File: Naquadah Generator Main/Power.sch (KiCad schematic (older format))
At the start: 12 parts, among them J10 Power Board Conn, J9 Power_Conn, Q1 30V 5A

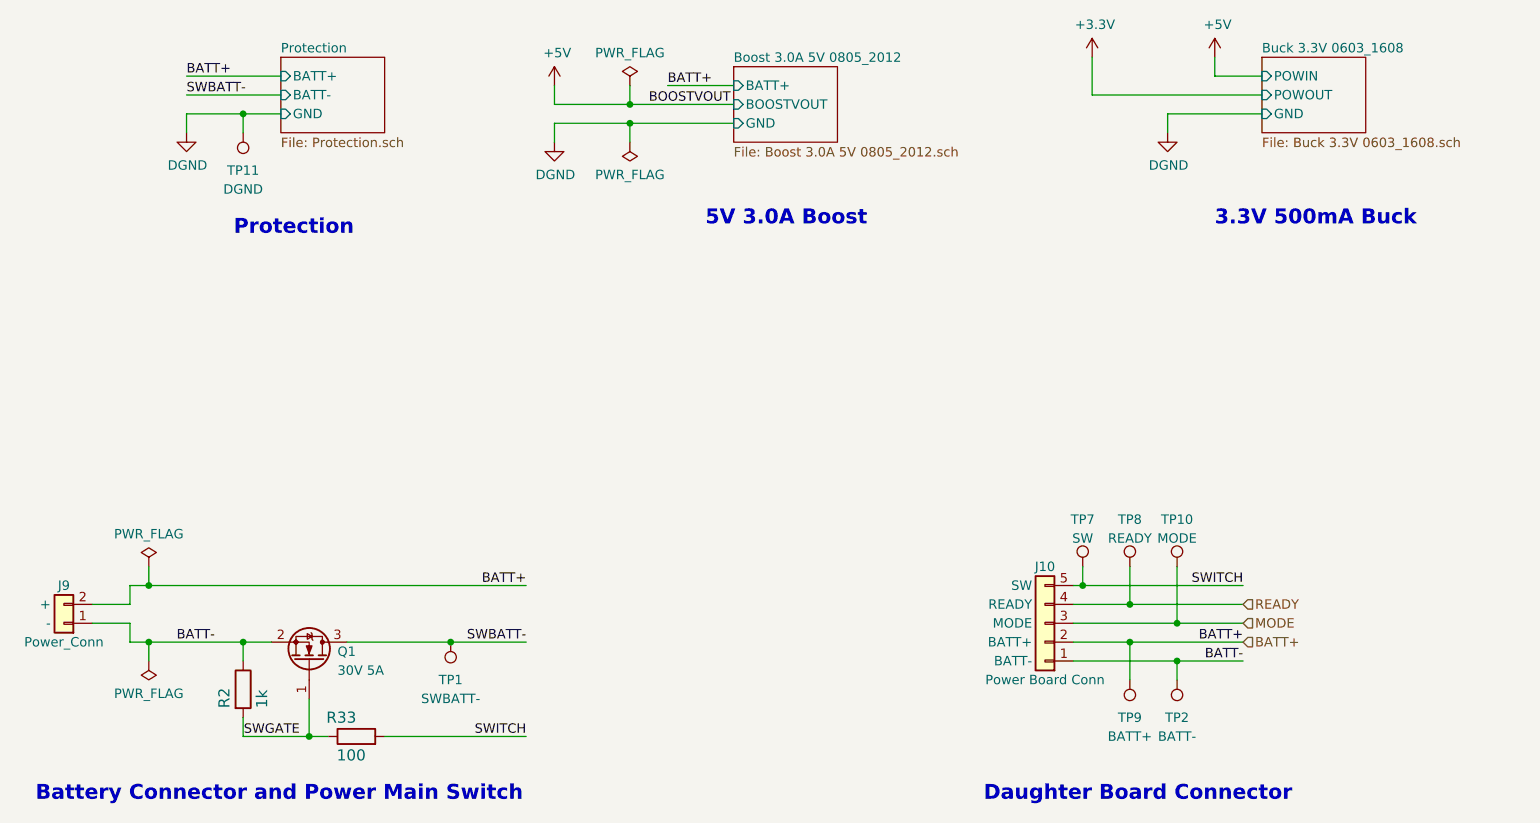
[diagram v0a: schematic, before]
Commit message: Added level shifter, moved user interface connector location
Added level shifter, moved user interface connector location
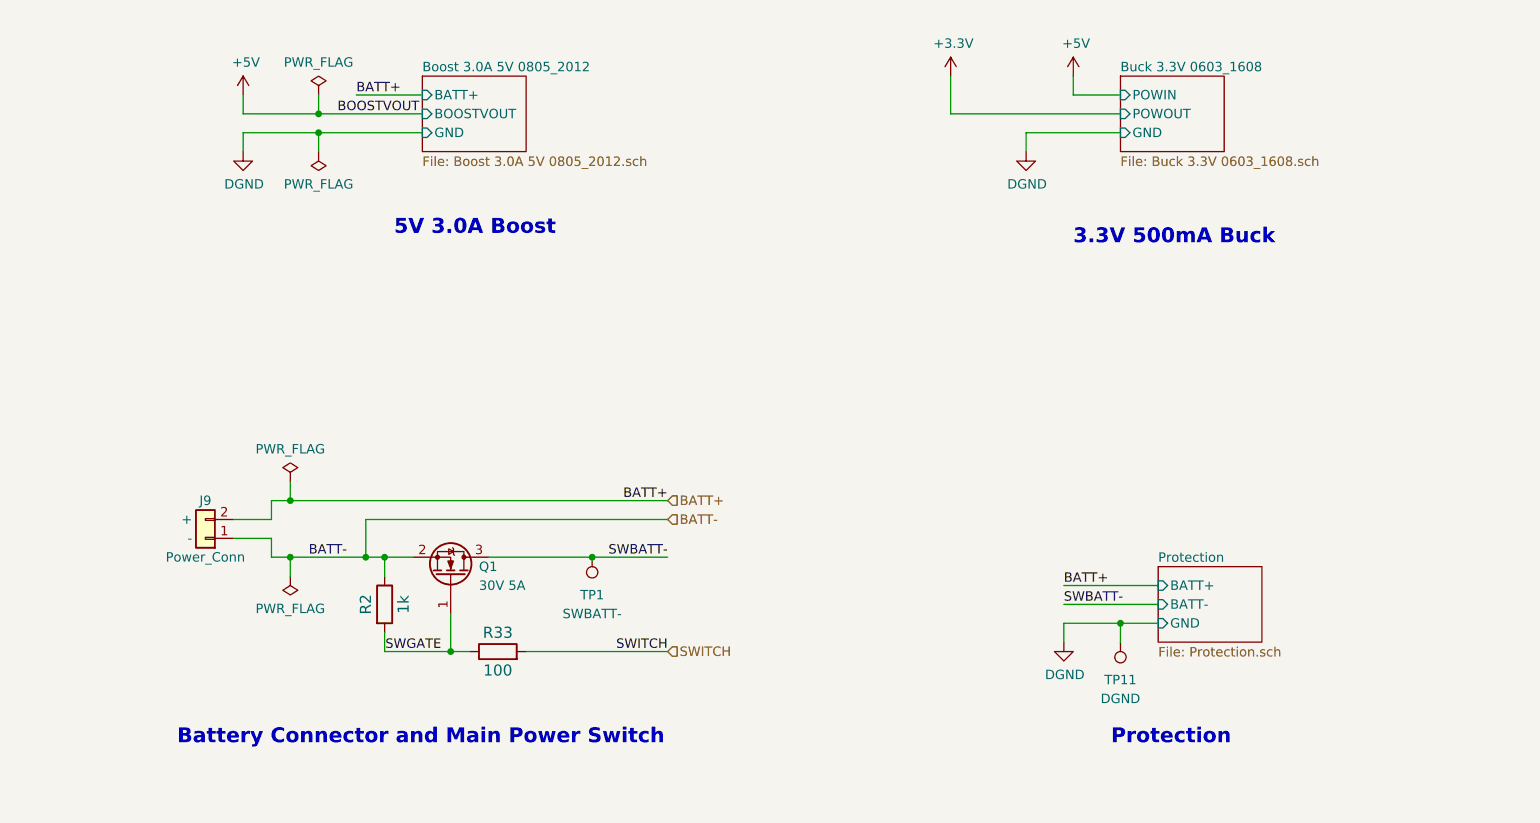
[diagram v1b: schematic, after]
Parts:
- removed J10: Power Board Conn, Naquadah_Generator:Daughter_Board_Vert_5_Pin_JST_Conn, symbol Naquadah_Generator:Power_Daughter_5_Pin_Conn
- removed TP10, TP2, TP7, TP8, TP9: TestPoint, Frequently_Used_LE:Pad_2.5-2.5, symbol Frequently_Used_LE:TestPoint_1
- R2: footprint Frequently_Used_LE:0805_2012Metric_HandSolder -> Frequently_Used_LE:0805_2012Metric
- R33: footprint Frequently_Used_LE:0805_2012Metric_HandSolder -> Frequently_Used_LE:0805_2012Metric; Description 1 kOhms ±1% 0.25W, 1/4W Chip Resistor 1206 (3216 Metric) -> 100 Ohms ±1% 0.25W, 1/4W Chip Resistor 0805 (2012 Metric) A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; Manufacturer Part No. RK73H2ATTD1001F -> RK73H2ATTD1000F; Source Part No. 2019-RK73H2ATTD1001FCT-ND -> 2019-RK73H2ATTD1000FCT-ND
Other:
- note added: "Battery Connector and Main Power Switch"
- note removed: "Battery Connector and Power Main Switch"
- note removed: "Daughter Board Connector"
- moved on the sheet: J9, Q1, R2, R33, TP1, TP11

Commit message: Switched to 0603_1608M size for passives
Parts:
- J9: symbol Connectors_LE:Power_Conn -> Connector_LE:Power_Conn; Description (none) -> Battery Holder (Open) 18650 1 Cell SMD (SMT) Tab; Manufacturer Name (none) -> Keystone Electronics; Manufacturer Part No. (none) -> 1042; Source (none) -> Digikey; Source Part No. (none) -> 36-1042-ND
- R2: footprint Frequently_Used_LE:0805_2012Metric -> Frequently_Used_LE:0603_1608Metric; Description 1 kOhms ±1% 0.25W, 1/4W Chip Resistor 1206 (3216 Metric) -> 1 kOhms ±1% 0.25W, 1/4W Chip Resistor 0603 (1608 Metric) Au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; Manufacturer Name KOA Speer Electronics, Inc. -> Rohm Semiconductor; Manufacturer Part No. RK73H2ATTD1001F -> ESR03EZPF1001; Source Part No. 2019-RK73H2ATTD1001FCT-ND -> RHM1.00KADCT-ND
- R33: footprint Frequently_Used_LE:0805_2012Metric -> Frequently_Used_LE:0603_1608Metric; Description 100 Ohms ±1% 0.25W, 1/4W Chip Resistor 0805 (2012 Metric) A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 -> 100 Ohms ±1% 0.25W, 1/4W Chip Resistor 0603 (1608 Metric) A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; Manufacturer Name KOA Speer Electronics, Inc. -> Panasonic Electronic Components; Manufacturer Part No. RK73H2ATTD1000F -> ERJ-PA3F1000V; Source Part No. 2019-RK73H2ATTD1000FCT-ND -> P100BYCT-ND
- TP1, TP11: Description None -> Test point
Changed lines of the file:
@@
 $Descr A 11000 8500
 encoding utf-8
-Sheet 10 17
+Sheet 10 18
 Title "Li-ion 3A Boost 1A Charge Protect"
 Date ""
@@
 F 0 "R33" V 4000 5250 59  0000 C CNN
 F 1 "100" V 3800 5250 59  0000 C CNN
-F 2 "Frequently_Used_LE:0805_2012Metric" H 3900 5250 50  0001 C CNN
-F 3 "http://www.koaspeer.com/pdfs/RK73H.pdf" H 3900 5250 50  0001 C CNN
-F 4 "100 Ohms ±1% 0.25W, 1/4W Chip Resistor 0805 (2012 Metric) Automotive AEC-Q200, Moisture Resistant Thick Film" H 3900 5250 50  0001 C CNN "Description"
-F 5 "2019-RK73H2ATTD1000FCT-ND" H 3900 5250 50  0001 C CNN "Source Part No."
-F 6 "RK73H2ATTD1000F" H 3900 5250 50  0001 C CNN "Manufacturer Part No."
-F 7 "KOA Speer Electronics, Inc." H 3900 5250 50  0001 C CNN "Manufacturer Name"
+F 2 "Frequently_Used_LE:0603_1608Metric" H 3900 5250 50  0001 C CNN
+F 3 "https://industrial.panasonic.com/cdbs/www-data/pdf/RDO0000/AOA0000C331.pdf" H 3900 5250 50  0001 C CNN
+F 4 "100 Ohms ±1% 0.25W, 1/4W Chip Resistor 0603 (1608 Metric) Automotive AEC-Q200, Pulse Withstanding Thick Film" H 3900 5250 50  0001 C CNN "Description"
+F 5 "P100BYCT-ND" H 3900 5250 50  0001 C CNN "Source Part No."
+F 6 "ERJ-PA3F1000V" H 3900 5250 50  0001 C CNN "Manufacturer Part No."
+F 7 "Panasonic Electronic Components" H 3900 5250 50  0001 C CNN "Manufacturer Name"
 F 8 "Digikey" H 3900 5250 50  0001 C CNN "Source"
 	1    3900 5250
@@
 F 0 "R2" V 3200 5000 59  0000 C CNN
 F 1 "1k" V 3400 5000 59  0000 C CNN
-F 2 "Frequently_Used_LE:0805_2012Metric" H 3300 5000 50  0001 C CNN
-F 3 "http://www.koaspeer.com/pdfs/RK73H.pdf" H 3300 5000 50  0001 C CNN
-F 4 "1 kOhms ±1% 0.25W, 1/4W Chip Resistor 1206 (3216 Metric) " H 3300 5000 50  0001 C CNN "Description"
-F 5 "2019-RK73H2ATTD1001FCT-ND" H 3300 5000 50  0001 C CNN "Source Part No."
-F 6 "RK73H2ATTD1001F" H 3300 5000 50  0001 C CNN "Manufacturer Part No."
-F 7 "KOA Speer Electronics, Inc." H 3300 5000 50  0001 C CNN "Manufacturer Name"
+F 2 "Frequently_Used_LE:0603_1608Metric" H 3300 5000 50  0001 C CNN
+F 3 "https://d1d2qsbl8m0m72.cloudfront.net/en/products/databook/datasheet/passive/resistor/chip_resistor/esr-e.pdf" H 3300 5000 50  0001 C CNN
+F 4 "1 kOhms ±1% 0.25W, 1/4W Chip Resistor 0603 (1608 Metric) Automotive AEC-Q200, Pulse Withstanding Thick Film" H 3300 5000 50  0001 C CNN "Description"
+F 5 "RHM1.00KADCT-ND" H 3300 5000 50  0001 C CNN "Source Part No."
+F 6 "ESR03EZPF1001" H 3300 5000 50  0001 C CNN "Manufacturer Part No."
+F 7 "Rohm Semiconductor" H 3300 5000 50  0001 C CNN "Manufacturer Name"
 F 8 "Digikey" H 3300 5000 50  0001 C CNN "Source"
 	1    3300 5000
@@
 	2500 4650 2700 4650
 $Comp
-L Connectors_LE:Power_Conn J9
+L Connector_LE:Power_Conn J9
 U 1 1 5EE056F1
 P 2350 4650
@@
 F 1 "Power_Conn" H 2350 4750 50  0000 C CNN
 F 2 "Naquadah_Generator:Keystone-1042" H 2350 4650 50  0001 C CNN
-F 3 "~" H 2350 4650 50  0001 C CNN
+F 3 "https://www.keyelco.com/userAssets/file/M65p27.pdf" H 2350 4650 50  0001 C CNN
+F 4 "Battery Holder (Open) 18650 1 Cell SMD (SMT) Tab" H 2350 4650 50  0001 C CNN "Description"
+F 5 "Keystone Electronics" H 2350 4650 50  0001 C CNN "Manufacturer Name"
+F 6 "1042" H 2350 4650 50  0001 C CNN "Manufacturer Part No."
+F 7 "Digikey" H 2350 4650 50  0001 C CNN "Source"
+F 8 "36-1042-ND" H 2350 4650 50  0001 C CNN "Source Part No."
 	1    2350 4650
 	-1   0    0    1
@@
 F 7 "None" H 7195 4845 50  0001 C CNN "Manufacturer Name"
 F 8 "None" H 7195 4845 50  0001 C CNN "Manufacturer Part No."
-F 9 "None" H 7200 5200 50  0001 C CNN "Description"
+F 9 "Test point" H 7200 5200 50  0001 C CNN "Description"
 	1    7200 5200
 	-1   0    0    1
@@
 F 3 "None" H 4600 4750 50  0001 C CNN
 F 4 "SWBATT-" H 4400 5050 50  0000 C CNN "Name"
-F 5 "None" H 4400 4750 50  0001 C CNN "Description"
+F 5 "Test point" H 4400 4750 50  0001 C CNN "Description"
 F 6 "None" H 4400 4750 50  0001 C CNN "Source Part No."
 F 7 "None" H 4400 4750 50  0001 C CNN "Manufacturer Name"
